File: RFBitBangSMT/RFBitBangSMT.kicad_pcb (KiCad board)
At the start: 2 copper layers, 152 x 88 mm, 260 parts, among them J1 POWER, J10 si5351mod, J11 AudioJack2_Dual_Ground_Switch, J12 Conn_Coaxial, J13 Conn_01x01, J14 Conn_01x01, J15 Conn_01x01, J16 Conn_01x01, J17 Filt1, J18 Filt2, J19 AudioJack2_Dual_Ground_Switch, J2 Barrel_Jack, J20 Conn_01x01, J21 Conn_01x01, J3 Conn_01x01, J4 Conn_01x01, J5 Conn_01x04, J6 Conn_01x01, J7 Conn_01x01, J8 AudioJack2_Dual_Ground_Switch, J9 ICSP, P1 Mini-DIN_6pins_ver4, Q1 MMBT3904, Q10 MMBT3904, Q11 MMBT3904, Q12 MMBT3904, Q13 SS8550, Q14 MMBT3904, Q15 NC, Q16 SS8550, Q2 MMBT3904, Q3 2N7000, Q4 MMBT3904, Q5 NC, Q6 2N7000, Q7 2N7000, Q8 SS8550, Q9 2N7000, SW1 SW_Push, SW2 SW_Push, SW3 SW_Push, SW4 SW_Push, SW5 SW_Push, SW6 SW_Push, T1 Trifilar, T2 Trifilar, T3 Current, T4 Common-Mode Choke, U1 ATmega328P-A, U2 LM78M05_TO252, U3 LM386, U4 LM358, U5 LM358, U6 SI5351A, Y1 16 MHz, Y2 7.X MHz, Y3 25 MHz, Y4 7.X MHz, Y5 7.X MHz

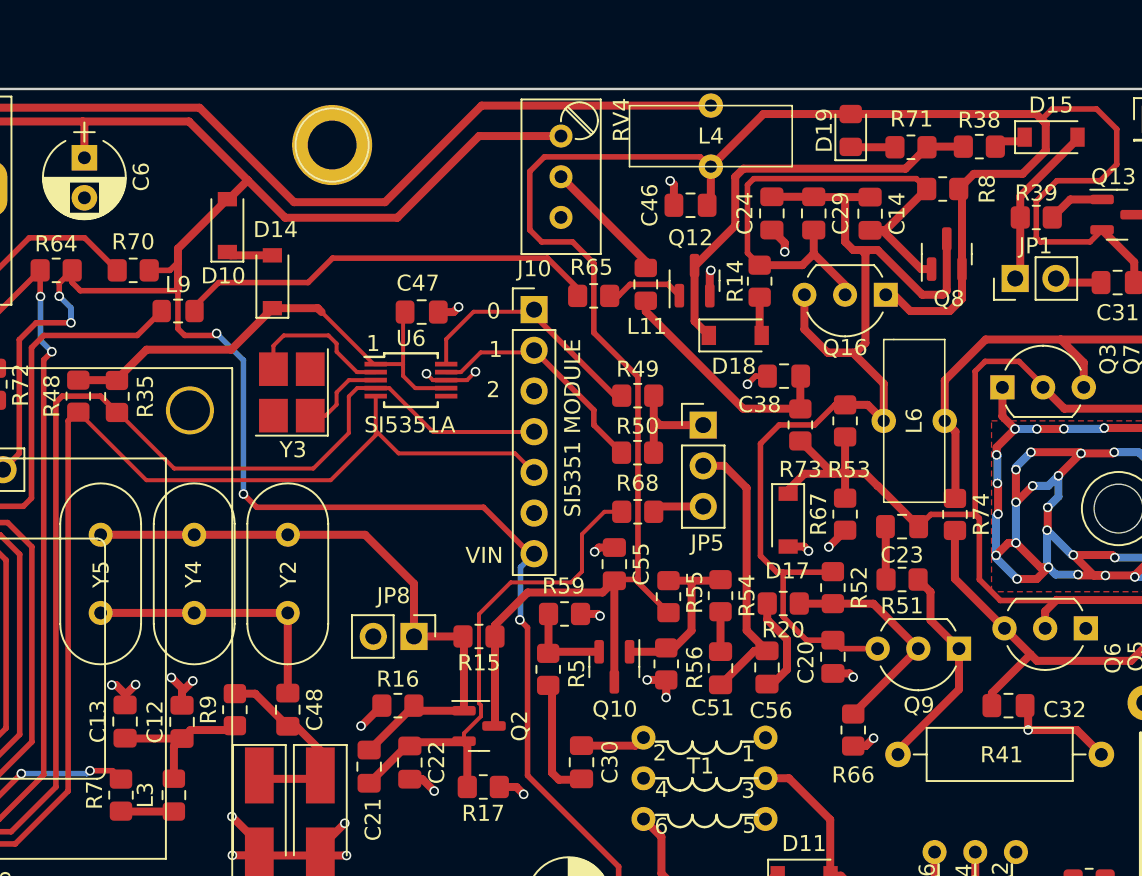
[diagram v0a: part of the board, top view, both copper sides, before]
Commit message: Added Low Pass Filter
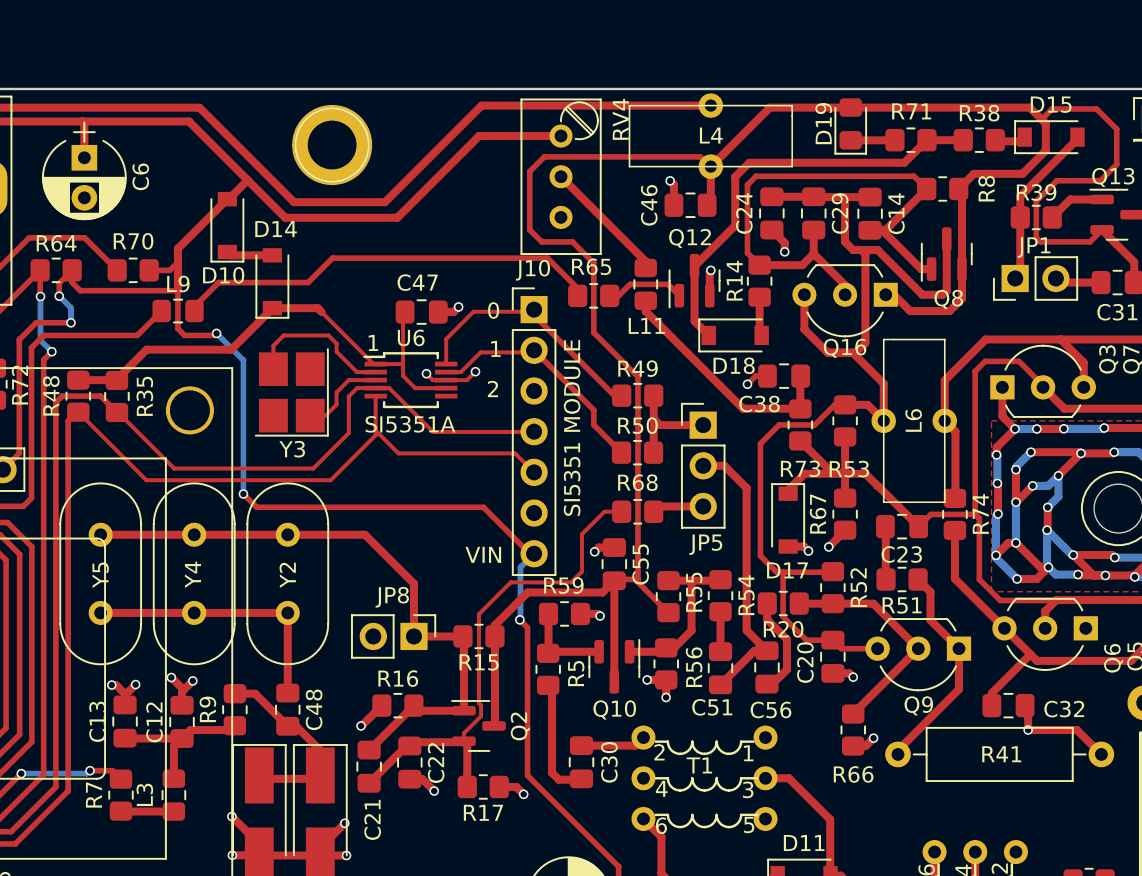
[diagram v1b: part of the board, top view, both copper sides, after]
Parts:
- moved R71 0.44 mm to (164.6, 60.2)
- moved D19 0.41 mm to (160.9, 59.2)
- moved R38 0.40 mm to (168.9, 60.2)

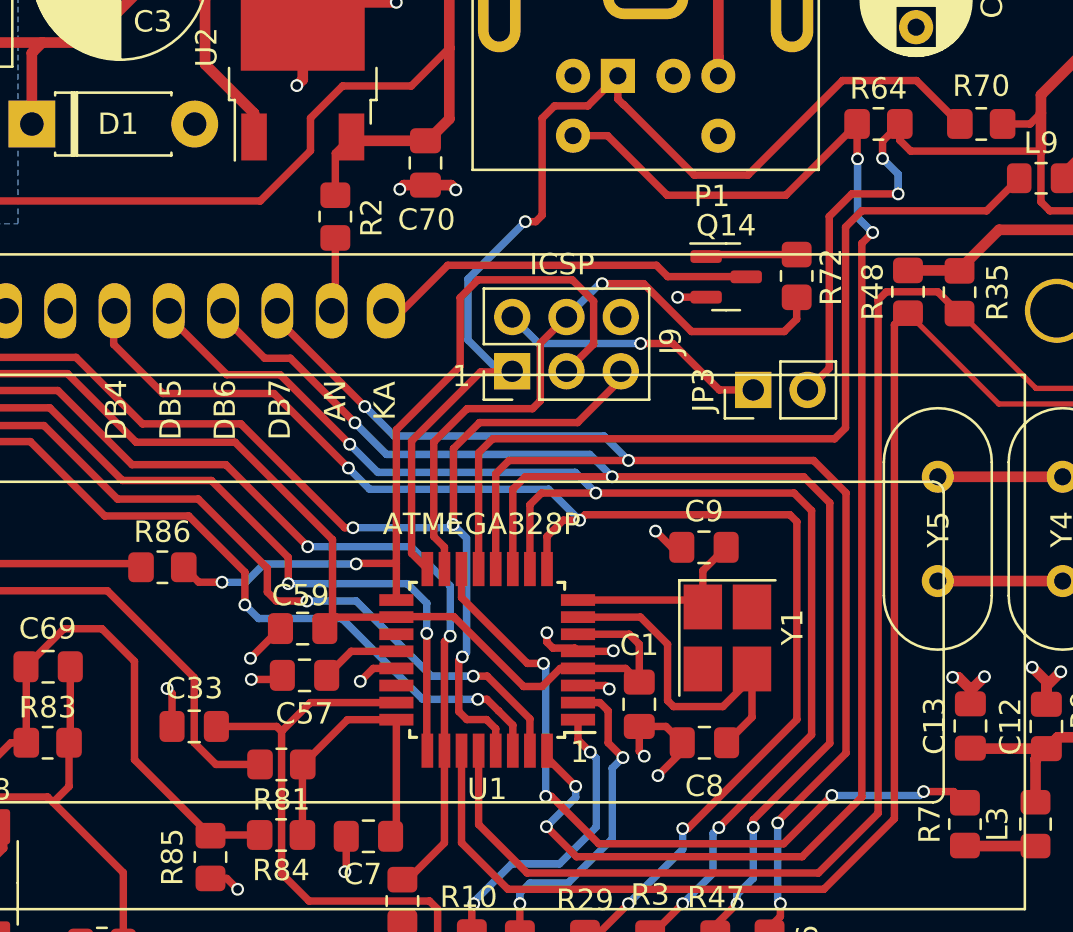
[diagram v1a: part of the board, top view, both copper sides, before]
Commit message: JLCPCB order
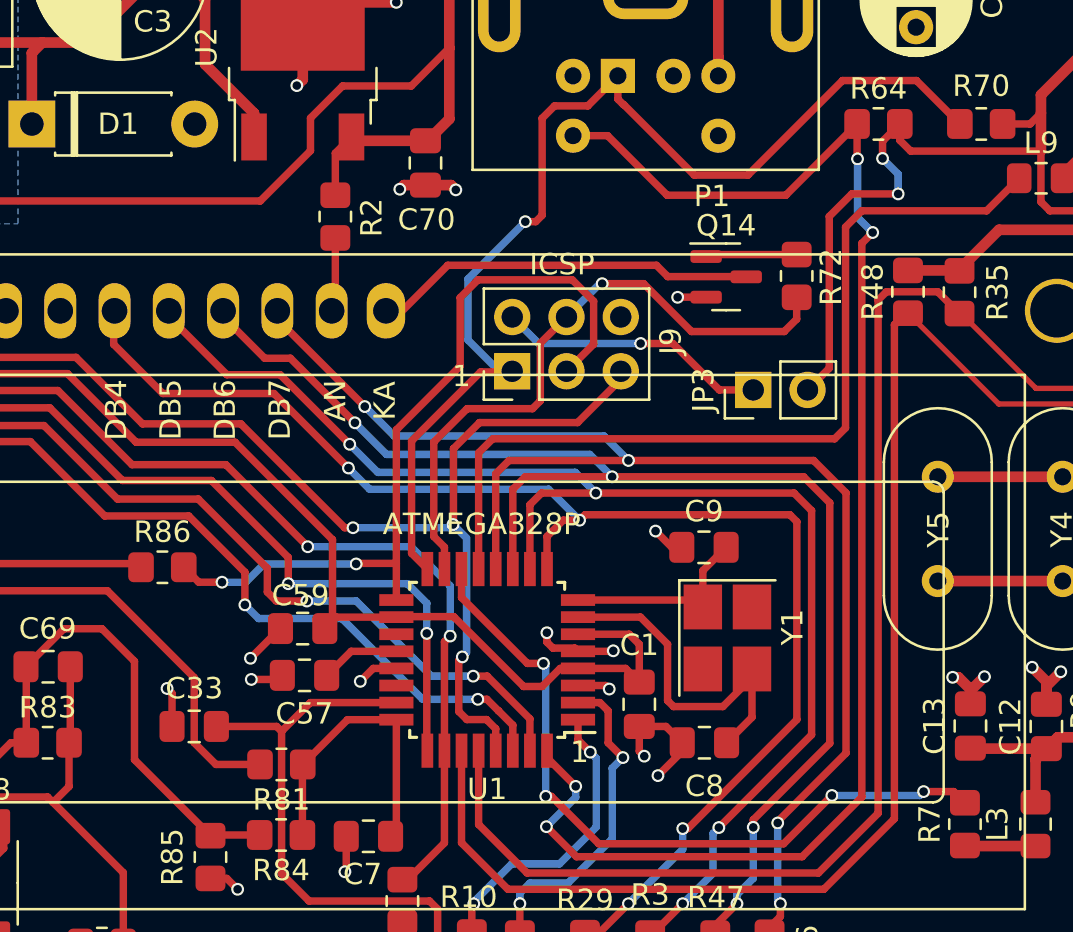
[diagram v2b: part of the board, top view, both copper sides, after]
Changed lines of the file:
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@@
     (fp_arc (start 0.20066 22.9997) (mid -0.153162 22.853142) (end -0.29972 22.49932) (layer "F.SilkS") (width 0.12))
     (fp_arc (start 63.7 8) (mid 64.053553 8.146447) (end 64.2 8.5) (layer "F.SilkS") (width 0.12))
-    (fp_arc (start 64.20104 22.49932) (mid 64.054479 22.85315) (end 63.70066 22.9997) (layer "F.SilkS") (width 0.12))
+    (fp_arc (start 64.20104 22.49932) (mid 64.054473 22.853115) (end 63.70066 22.9997) (layer "F.SilkS") (width 0.12))
     (fp_arc (start -0.29972 8.49884) (mid -0.153162 8.145018) (end 0.20066 7.99846) (layer "F.SilkS") (width 0.12))
     (fp_line (start -8.25 -2.75) (end 72.25 -2.75) (layer "F.CrtYd") (width 0.05))
@@
     (fp_line (start -1 0.625) (end -1 -0.625) (layer "F.Fab") (width 0.1))
     (fp_line (start 1 0.625) (end -1 0.625) (layer "F.Fab") (width 0.1))
-    (pad "1" smd roundrect (at -1.0375 0 90) (size 1.175 1.45) (layers "F.Cu" "F.Paste" "F.Mask") (roundrect_rratio 0.212766)
+    (pad "1" smd roundrect (at -1.0375 0 90) (size 1.175 1.45) (layers "F.Cu" "F.Paste" "F.Mask") (roundrect_rratio 0.2127659574)
       (net 2 "GND") (pintype "passive"))
-    (pad "2" smd roundrect (at 1.0375 0 90) (size 1.175 1.45) (layers "F.Cu" "F.Paste" "F.Mask") (roundrect_rratio 0.212766)
+    (pad "2" smd roundrect (at 1.0375 0 90) (size 1.175 1.45) (layers "F.Cu" "F.Paste" "F.Mask") (roundrect_rratio 0.2127659574)
       (net 1 "+5V") (pintype "passive"))
     (model "${KICAD6_3DMODEL_DIR}/Capacitor_SMD.3dshapes/C_0805_2012Metric.wrl"
@@
     (fp_line (start -1 0.625) (end -1 -0.625) (layer "F.Fab") (width 0.1))
     (fp_line (start -1 -0.625) (end 1 -0.625) (layer "F.Fab") (width 0.1))
-    (pad "1" smd roundrect (at -1 0) (size 1.2 1.4) (layers "F.Cu" "F.Paste" "F.Mask") (roundrect_rratio 0.208333)
+    (pad "1" smd roundrect (at -1 0) (size 1.2 1.4) (layers "F.Cu" "F.Paste" "F.Mask") (roundrect_rratio 0.2083333333)
       (net 163 "Net-(R80-Pad1)") (pintype "passive"))
-    (pad "2" smd roundrect (at 1 0) (size 1.2 1.4) (layers "F.Cu" "F.Paste" "F.Mask") (roundrect_rratio 0.208333)
+    (pad "2" smd roundrect (at 1 0) (size 1.2 1.4) (layers "F.Cu" "F.Paste" "F.Mask") (roundrect_rratio 0.2083333333)
       (net 17 "SCK") (pintype "passive"))
     (model "${KICAD6_3DMODEL_DIR}/Resistor_SMD.3dshapes/R_0805_2012Metric.wrl"
